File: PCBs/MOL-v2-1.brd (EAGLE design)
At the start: 139.7 x 50.8 mm, 24 parts, among them IC1 ULN2803, IC2 ULN2803, J1 SERVO1, J2 SERVO2, J3 STRIPS, J4 ACTUATORS

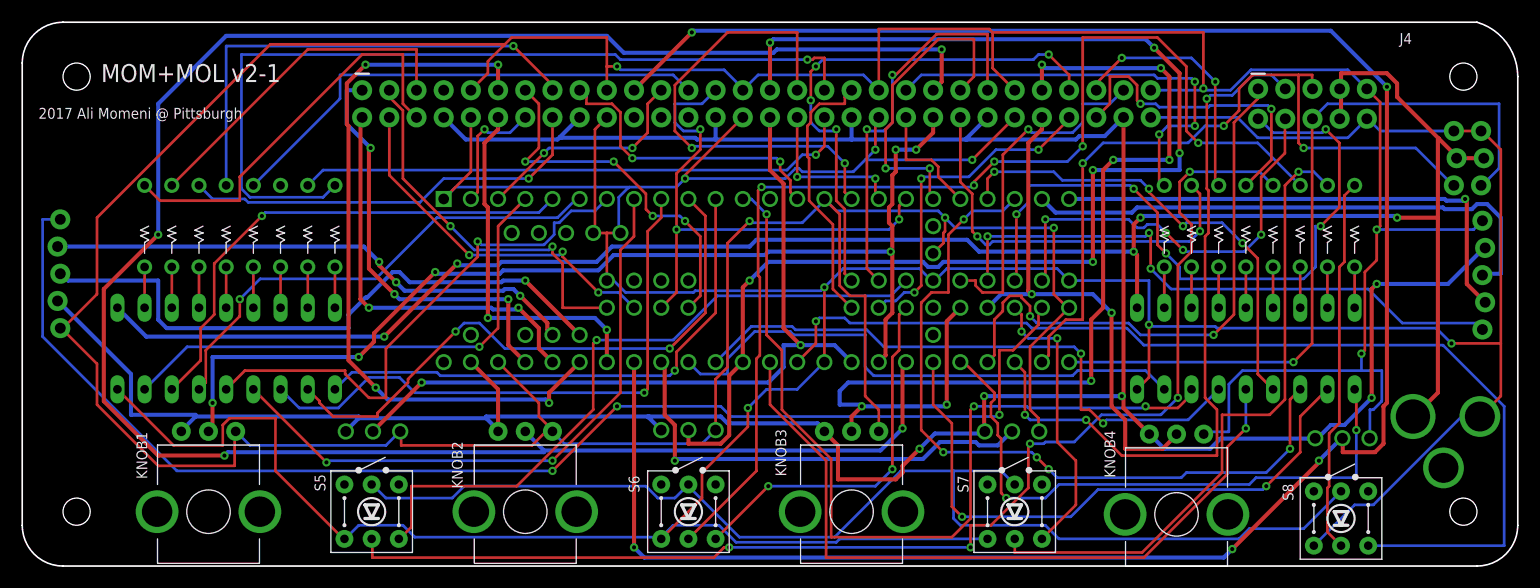
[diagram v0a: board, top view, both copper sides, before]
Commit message: reroute + Arduino stuff
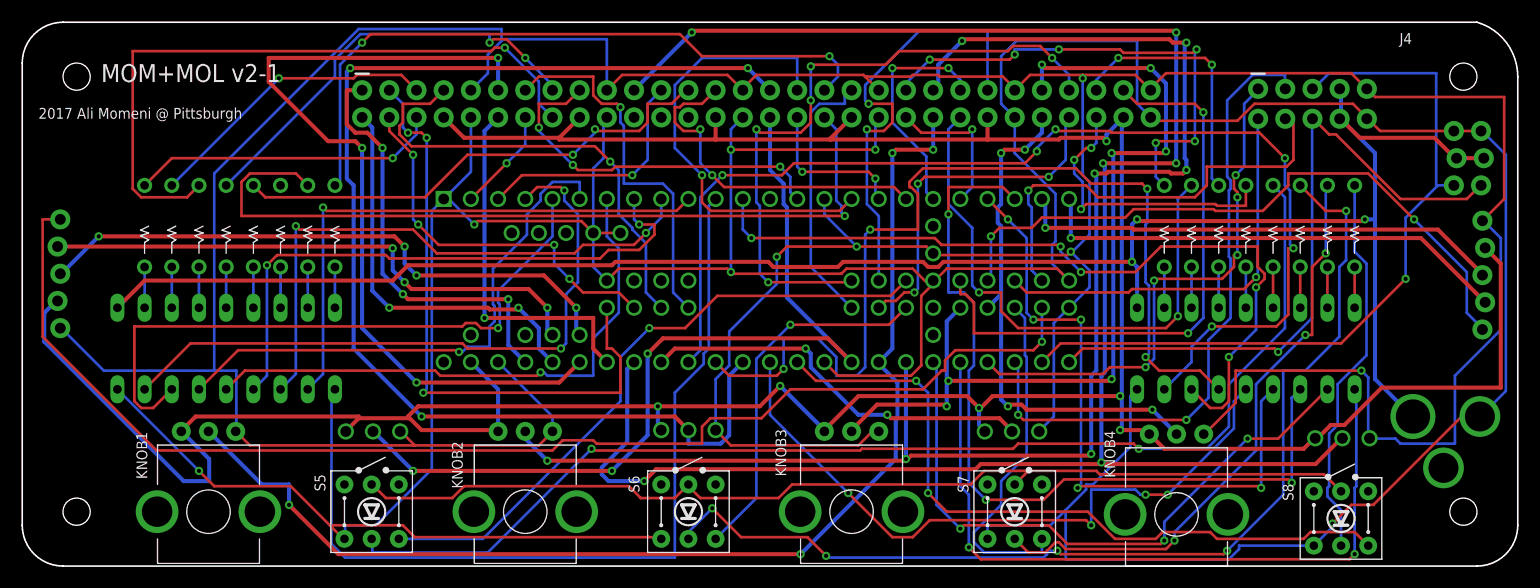
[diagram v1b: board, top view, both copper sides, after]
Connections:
- net LED1: now also U$3.55
- net LED3: no longer U$3.55
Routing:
- net AN10: track 197.3 -> 137.9 mm, vias 4 -> 7
- net PWM10: track 51.8 -> 105.1 mm, vias 0 -> 6
- net LED1: track 0.00 -> 43.7 mm, vias 0 -> 1
- net PWM11: track 56.5 -> 90.4 mm, vias 2 -> 4
- net PWM7: track 50.3 -> 82.2 mm, vias 1 -> 0
- net B16: track 98.1 -> 67.0 mm, vias 1 -> 2
- net M_AIN: track 64.3 -> 38.5 mm, vias 5 -> 1
- net PWM_4: track 39.0 -> 63.1 mm
- net PWM_8: track 52.5 -> 76.5 mm
- net AGND: track 282.5 -> 305.3 mm, vias 5 -> 6
- net +3V3: track 426.6 -> 403.9 mm, vias 7 -> 5
- net LED6: track 32.6 -> 55.3 mm, vias 1 -> 2
- net B1: track 35.9 -> 57.7 mm, vias 2 -> 3
- net AN5: track 202.3 -> 183.2 mm, vias 5 -> 6
- net LED3: track 50.4 -> 32.4 mm, vias 3 -> 2
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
